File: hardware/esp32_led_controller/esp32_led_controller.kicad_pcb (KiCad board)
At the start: 4 copper layers, 114 x 153 mm, 565 parts, among them J1 USB_B, J2 CONN_01X09, J3 CONN_01X05, J4 BARREL_JACK, J5 CONN_01X03, J6 USB_C_Receptacle_USB2.0, Q1 Q_NPN_BEC, Q2 Q_NPN_BEC, SW1 SW_Push, U1 MCP1415, U2 CP2102, U3 ESP32-WROOM-32, U4 AZ1117-3.3

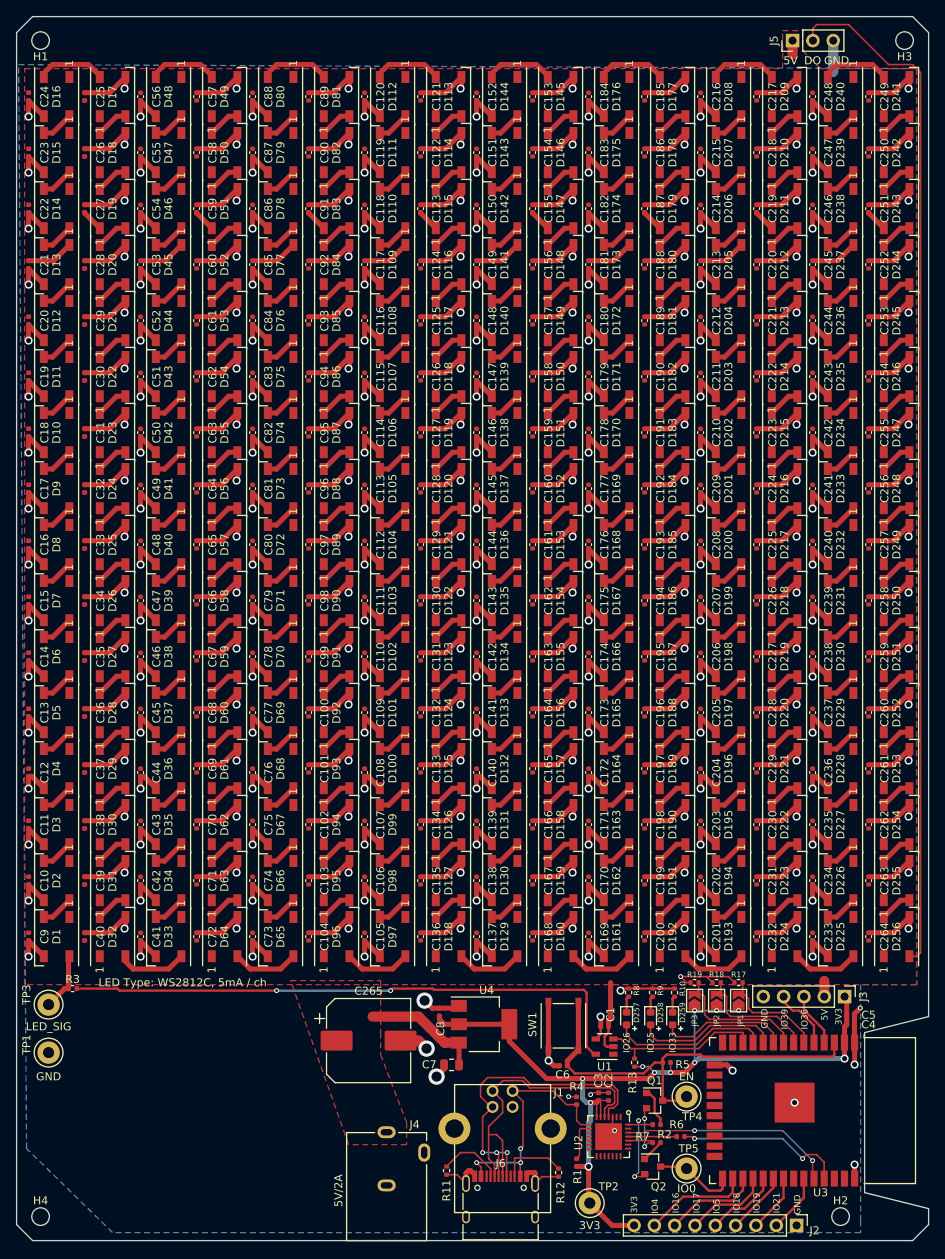
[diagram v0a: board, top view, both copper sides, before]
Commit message: Added rev4 hardware design
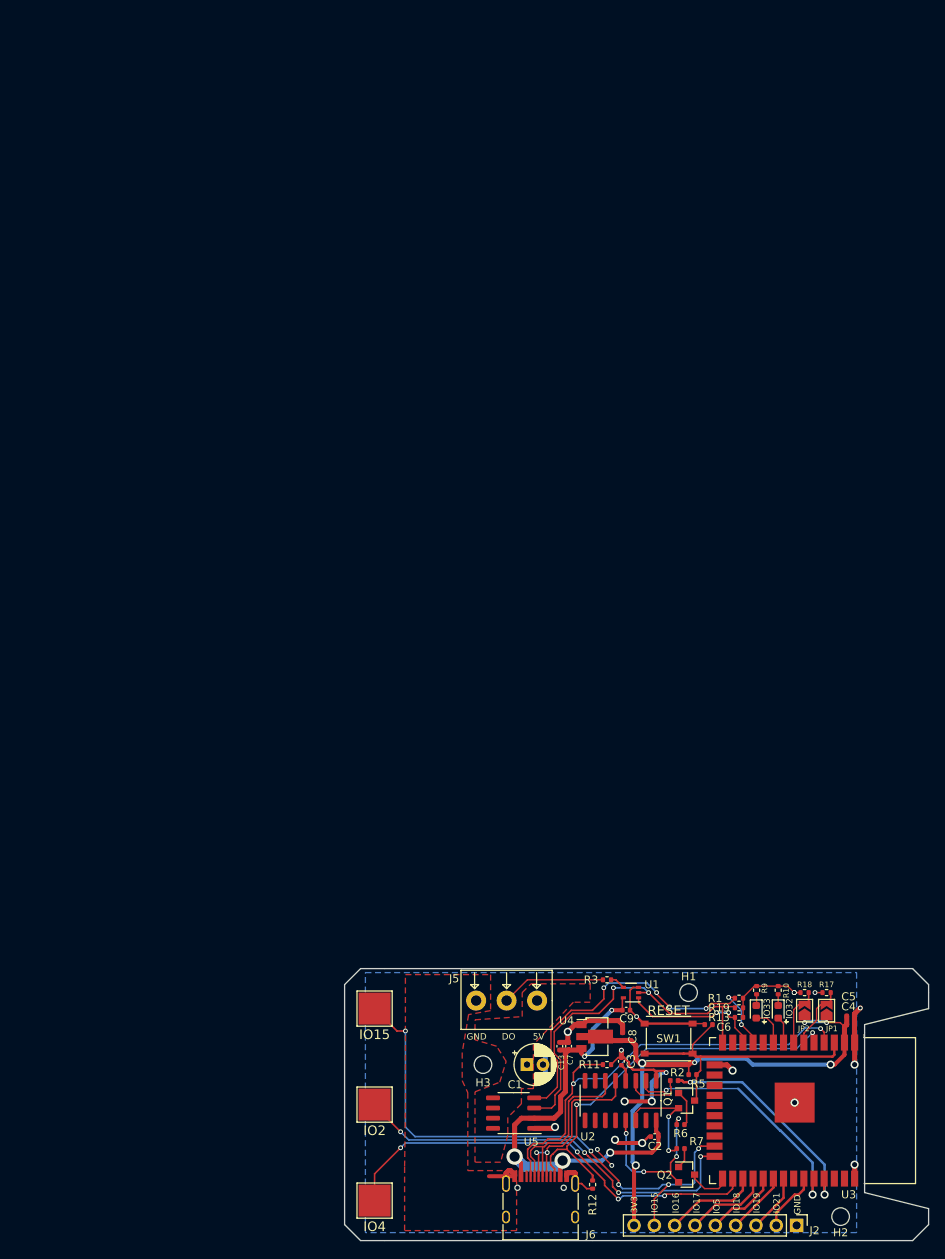
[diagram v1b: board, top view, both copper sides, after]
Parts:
- removed C10, C100, C101, C102, C103, C104, C105, C106, C107, C108, C109, C11, C110, C111, C112, C113, C114, C115, C116, C117, C118, C119, C12, C120, C121, C122, C123, C124, C125, C126, C127, C128, C129, C130, C131, C132, C133, C134, C135, C136, C137, C138, C139, C14, C140, C141, C142, C143, C144, C145, C146, C147, C148, C149, C15, C150, C151, C152, C153, C154, C155, C156, C157, C158, C159, C16, C160, C161, C162, C163, C164, C165, C166, C167, C168, C169, C17, C170, C171, C172, C173, C174, C175, C176, C177, C178, C179, C18, C180, C181, C182, C183, C184, C185, C186, C187, C188, C189, C19, C190, C191, C192, C193, C194, C195, C196, C197, C198, C199, C20, C200, C201, C202, C203, C204, C205, C206, C207, C208, C209, C21, C210, C211, C212, C213, C214, C215, C216, C217, C218, C219, C22, C220, C221, C222, C223, C224, C225, C226, C227, C228, C229, C23, C230, C231, C232, C233, C234, C235, C236, C237, C238, C239, C24, C240, C241, C242, C243, C244, C245, C246, C247, C248, C249, C25, C250, C251, C252, C253, C254, C255, C256, C257, C258, C259, C26, C260, C261, C262, C263, C264, C27, C28, C29, C30, C31, C32, C33, C34, C35, C36, C37, C38, C39, C40, C41, C42, C43, C44, C45, C46, C47, C48, C49, C50, C51, C52, C53, C54, C55, C56, C57, C58, C59, C60, C61, C62, C63, C64, C65, C66, C67, C68, C69, C70, C71, C72, C73, C74, C75, C76, C77, C78, C79, C80, C81, C82, C83, C84, C85, C86, C87, C88, C89, C90, C91, C92, C93, C94, C95, C96, C97, C98, C99: 0.1uF, Capacitor_SMD:C_0402_1005Metric
- removed C265: 1000uF, Capacitor_SMD:CP_Elec_10x10
- removed D1, D10, D100, D101, D102, D103, D104, D105, D106, D107, D108, D109, D11, D110, D111, D112, D113, D114, D115, D116, D117, D118, D119, D12, D120, D121, D122, D123, D124, D125, D126, D127, D128, D129, D13, D130, D131, D132, D133, D134, D135, D136, D137, D138, D139, D14, D140, D141, D142, D143, D144, D145, D146, D147, D148, D149, D15, D150, D151, D152, D153, D154, D155, D156, D157, D158, D159, D16, D160, D161, D162, D163, D164, D165, D166, D167, D168, D169, D17, D170, D171, D172, D173, D174, D175, D176, D177, D178, D179, D18, D180, D181, D182, D183, D184, D185, D186, D187, D188, D189, D19, D190, D191, D192, D193, D194, D195, D196, D197, D198, D199, D2, D20, D200, D201, D202, D203, D204, D205, D206, D207, D208, D209, D21, D210, D211, D212, D213, D214, D215, D216, D217, D218, D219, D22, D220, D221, D222, D223, D224, D225, D226, D227, D228, D229, D23, D230, D231, D232, D233, D234, D235, D236, D237, D238, D239, D24, D240, D241, D242, D243, D244, D245, D246, D247, D248, D249, D25, D250, D251, D252, D253, D254, D255, D256, D26, D27, D28, D29, D3, D30, D31, D32, D33, D34, D35, D36, D37, D38, D39, D4, D40, D41, D42, D43, D44, D45, D46, D47, D48, D49, D5, D50, D51, D52, D53, D54, D55, D56, D57, D58, D59, D6, D60, D61, D62, D63, D64, D65, D66, D67, D68, D69, D7, D70, D71, D72, D73, D74, D75, D76, D77, D78, D79, D8, D80, D81, D82, D83, D84, D85, D86, D87, D88, D89, D9, D90, D91, D92, D93, D94, D95, D96, D97, D98, D99: WS2812B, LED_SMD:LED_WS2812B_PLCC4_5.0x5.0mm_P3.2mm
- removed D257: R, LED_SMD:LED_0603_1608Metric
- removed the H3 at (239.0, 49.0)
- removed J1: USB_B, Amphenol:Amphenol_61729_0010BLF
- removed J3: CONN_01X05, Connector_PinHeader_2.54mm:PinHeader_1x05_P2.54mm_Vertical
- removed J4: BARREL_JACK, dc_jack:DC-005C-25A
- removed JP3: J_NO, Jumper:SolderJumper-2_P1.3mm_Open_TrianglePad1.0x1.5mm
- removed R4: 10kR, Resistor_SMD:R_0402_1005Metric
- removed R8: 100R, Resistor_SMD:R_0402_1005Metric
- removed TP3, TP4, TP5: TestPoint, TestPoint:TestPoint_Loop_D3.50mm_Drill1.4mm_Beaded
- added TP6: TestPoint, TestPoint:TestPoint_Pad_4.0x4.0mm, F.Cu at (172.8, 194.0)
- added U5: AP2172A, Package_SO:SO-8_3.9x4.9mm_P1.27mm, F.Cu at (190.1, 183.1)
- C1: value 1uF -> 470uF; footprint Capacitor_SMD:C_0402_1005Metric -> Capacitor_THT:CP_Radial_D5.0mm_P2.00mm
- C2: value 1uF -> 0.1uF
- C7: value 22uF -> 10uF; footprint Capacitor_SMD:C_0805_2012Metric -> Capacitor_SMD:C_0402_1005Metric
- J5: footprint Connector_PinHeader_2.54mm:PinHeader_1x03_P2.54mm_Vertical -> terminal_block:KF128L-3.81-3P
- TP1, TP2: footprint TestPoint:TestPoint_Loop_D3.50mm_Drill1.4mm_Beaded -> TestPoint:TestPoint_Pad_4.0x4.0mm
- U1: value MCP1415 -> SN74LV1T08; footprint Package_TO_SOT_SMD:SOT-23-5 -> Package_TO_SOT_SMD:SOT-353_SC-70-5
- U2: value CP2102 -> CH340B/CH340C; footprint Package_DFN_QFN:QFN-28-1EP_5x5mm_P0.5mm_EP3.35x3.35mm -> Package_SO:SOIC-16_3.9x9.9mm_P1.27mm
- U4: footprint Package_TO_SOT_SMD:SOT-223-3_TabPin2 -> Package_TO_SOT_SMD:SOT-89-3
- moved H1 144.0 mm to (212.0, 168.0)
- moved J5 125.2 mm to (189.2, 169.0), turned to 180 degrees
- moved C13 78.4 mm to (195.9, 174.7), turned to 90 degrees
- moved C9 75.3 mm to (204.2, 170.2), turned to 0 degrees
- moved R3 66.8 mm to (201.8, 166.4)
- moved H3 58.5 mm to (186.3, 177.0)
- moved TP1 41.1 mm to (172.8, 170.0)
- moved TP2 29.6 mm to (172.8, 182.0)
- moved R1 28.9 mm to (218.3, 168.7), turned to 180 degrees
- moved R11 24.0 mm to (201.8, 177.0), turned to 180 degrees
- moved C8 23.1 mm to (203.8, 173.5)
- moved C6 18.9 mm to (214.5, 172.0)
- moved C7 14.8 mm to (197.0, 174.7), turned to 90 degrees
- moved R13 14.2 mm to (218.3, 171.1), turned to 180 degrees
- moved U4 13.9 mm to (200.2, 173.5)
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- renumbered H4 to H3
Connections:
- C1 pad 1: +5V -> /LED_5V
- C2 pad 1: +3V3 -> +5V
- C3 pad 1: +3V3 -> Net-(C3-Pad1)
- D258 pad 2: /IO25 -> /IO33
- D259 pad 2: /IO33 -> /IO32
- J2 pad 8: /IO4 -> /IO15
- J5 pad 1: +5V -> /LED_5V
- J5 pad 2: /row7/Dout -> Net-(J5-Pad2)
- J6 pad A4: /Vbus -> +5V
- J6 pad A5: Net-(J6-PadA5) -> /CC1
- J6 pad A8: Net-(J6-PadA8) -> (no net)
- J6 pad A9: /Vbus -> +5V
- J6 pad B4: /Vbus -> +5V
- J6 pad B5: Net-(J6-PadB5) -> /CC2
- J6 pad B8: Net-(J6-PadB8) -> (no net)
- J6 pad B9: /Vbus -> +5V
- R1 pad 1: Net-(R1-Pad1) -> GND
- R1 pad 2: +3V3 -> /LED_ON1
- R11 pad 2: Net-(J6-PadA5) -> /CC1
- R12 pad 2: Net-(J6-PadB5) -> /CC2
- R13 pad 1: /DOUT -> GND
- R13 pad 2: +3V3 -> /DOUT
- R19 pad 2: /IO32 -> /LED_ON0
- R3 pad 1: /LED_SIG -> Net-(J5-Pad2)
- R3 pad 2: Net-(R3-Pad2) -> /LED_SIG
- TP1 pad 1: GND -> /IO15
- TP2 pad 1: +3V3 -> /IO2
- U1 pad 1: Net-(U1-Pad1) -> /DOUT
- U1 pad 2: +5V -> /LED_ON0
- U1 pad 3: /DOUT -> GND
- U1 pad 4: GND -> /LED_SIG
- U1 pad 5: Net-(R3-Pad2) -> +5V
- U2 pad 1: Net-(U2-Pad1) -> GND
- U2 pad 10: Net-(U2-Pad10) -> (no net)
- U2 pad 11: Net-(U2-Pad11) -> (no net)
- U2 pad 12: Net-(U2-Pad12) -> (no net)
- U2 pad 13: Net-(U2-Pad13) -> /USB_DTR
- U2 pad 14: Net-(U2-Pad14) -> /USB_RTS
- U2 pad 15: Net-(U2-Pad15) -> (no net)
- U2 pad 16: Net-(U2-Pad16) -> +5V
- U2 pad 2: Net-(U2-Pad2) -> /USB_TX
- U2 pad 3: GND -> /USB_RX
- U2 pad 4: /Dp -> Net-(C3-Pad1)
- U2 pad 5: /Dm -> /Dp
- U2 pad 6: +3V3 -> /Dm
- U2 pad 7: +3V3 -> (no net)
- U2 pad 8: /Vbus -> (no net)
- U2 pad 9: Net-(R1-Pad1) -> (no net)
- U3 pad 10: /IO25 -> (no net)
- U3 pad 11: /IO26 -> /LED_ON1
- U3 pad 13: Net-(U3-Pad13) -> (no net)
- U3 pad 14: Net-(U3-Pad14) -> /LED_ON0
- U3 pad 16: Net-(U3-Pad16) -> (no net)
- U3 pad 17: Net-(U3-Pad17) -> (no net)
- U3 pad 18: Net-(U3-Pad18) -> (no net)
- U3 pad 19: Net-(U3-Pad19) -> (no net)
- U3 pad 20: Net-(U3-Pad20) -> (no net)
- U3 pad 21: Net-(U3-Pad21) -> (no net)
- U3 pad 22: Net-(U3-Pad22) -> (no net)
- U3 pad 23: Net-(U3-Pad23) -> /IO15
- U3 pad 24: Net-(U3-Pad24) -> /IO2
- U3 pad 32: Net-(U3-Pad32) -> (no net)
- U3 pad 36: Net-(U3-Pad36) -> (no net)
- U3 pad 37: Net-(U3-Pad37) -> (no net)
- U3 pad 4: /IO36 -> /CC1
- U3 pad 5: /IO39 -> /CC2
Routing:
- net GND: track 1625.6 -> 92.0 mm, vias 271 -> 19
- net /row7/Dout: track 129.3 -> 0.00 mm
- net Net-(R3-Pad2): track 72.4 -> 0.00 mm, vias 2 -> 0
- net /IO15: track 0.00 -> 69.5 mm, vias 0 -> 5
- net /CC1: track 0.00 -> 56.9 mm, vias 0 -> 2
- net /CC2: track 0.00 -> 51.7 mm, vias 0 -> 2
- net /IO2: track 0.00 -> 51.7 mm, vias 0 -> 4
- net /LED_ON1: track 0.00 -> 46.8 mm, vias 0 -> 6
- net /LED_ON0: track 0.00 -> 45.8 mm, vias 0 -> 2
- net /IO4: track 13.2 -> 54.9 mm, vias 0 -> 4
- net +3V3: track 113.4 -> 74.1 mm, vias 11 -> 6
- net +5V: track 97.2 -> 60.0 mm, vias 0 -> 5
- net /Vbus: track 31.2 -> 0.00 mm, vias 3 -> 0
- net /IO26: track 19.8 -> 0.00 mm
- net /IO25: track 18.0 -> 0.00 mm
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- added copper zone on F.Cu, net /LED_5V
- added copper zone on F.Cu, net GND
- removed copper zone on F.Cu, net +5V
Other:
- board size 114 x 153 mm -> 73 x 34 mm
- board text added: "Blinkenlights Rev4"
- board text added: "IO15"
- board text added: "IO2"
- board text added: "IO32"
- board text added: "RESET"
- board text removed: "5V/2A"
- board text removed: "EN"
- board text removed: "ESP32LedControl Rev1"
- board text removed: "IO0"
- board text removed: "IO25"
- board text removed: "IO26"
- board text removed: "IO36"
- board text removed: "IO39"
- board text removed: "LED Type: WS2812C, 5mA / ch"
- board text removed: "LED_SIG"
